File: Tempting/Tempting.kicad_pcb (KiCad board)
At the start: 4 copper layers, 52.9 x 65 mm, 62 parts, among them J1 Conn_Coaxial, J2 Conn_01x07_Socket, J3 Conn_ARM_SWD_TagConnect_TC2030, J4 USB_C_Receptacle_USB2.0_16P, SW1 SPST, SW2 SPST, U1 AMS1117-3.3, U2 SCD41-D-R2, U3 STM32WB55CGUx, U4 DPS368, U5 USBLC6-2SC6, X1 32M, X2 32.768k

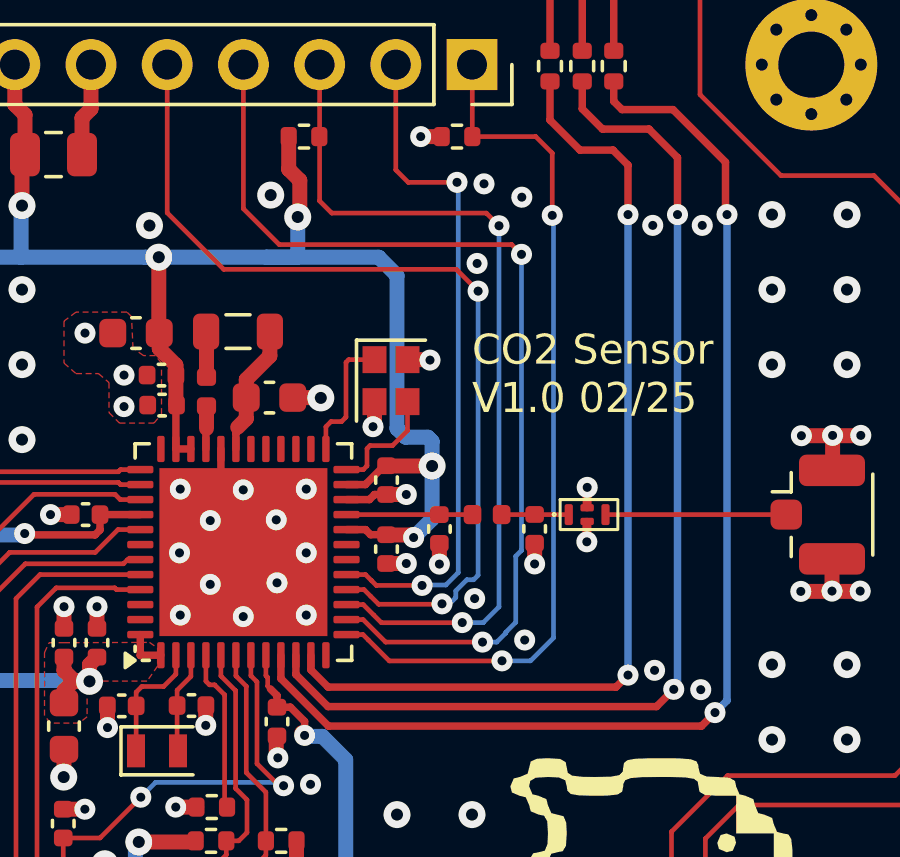
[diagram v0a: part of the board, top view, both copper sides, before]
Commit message: Updated gerbers
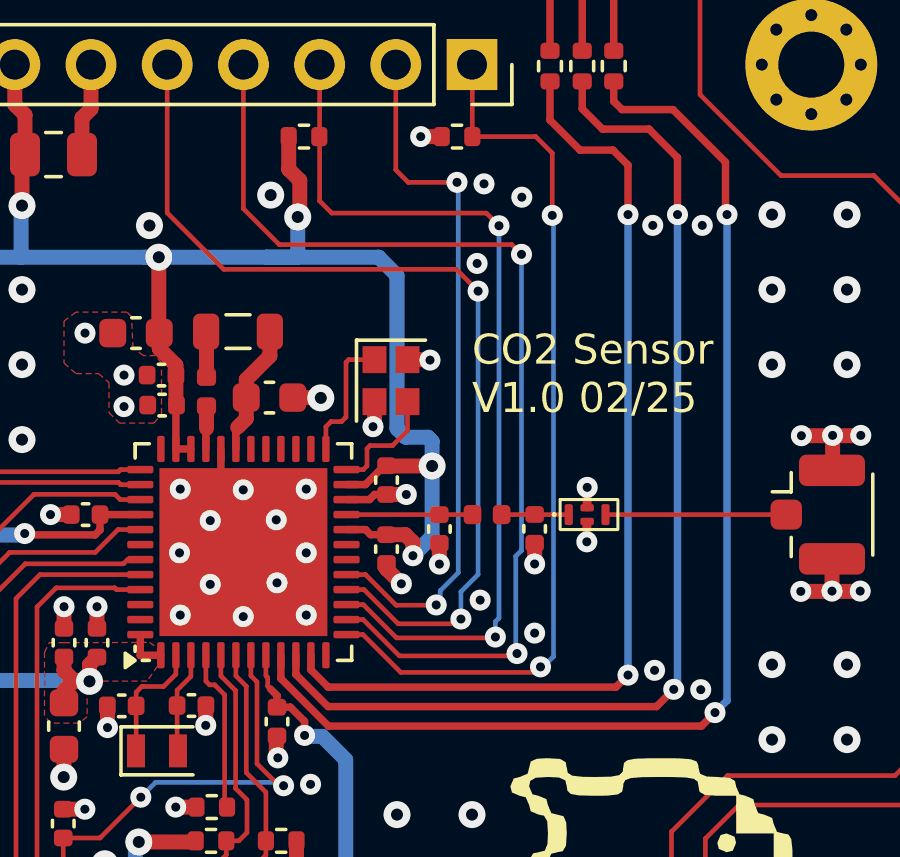
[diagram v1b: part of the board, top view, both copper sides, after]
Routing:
- net +3.3V: track 218.5 -> 219.6 mm
- net /OLED_CLK: track 33.3 -> 34.3 mm
- net /OLED_NCS: track 29.1 -> 30.1 mm
- net /OLED_DIN: track 31.0 -> 31.9 mm
- net /OLED_DC: track 22.8 -> 23.5 mm
- net /OLED_NRST: track 29.1 -> 29.7 mm
